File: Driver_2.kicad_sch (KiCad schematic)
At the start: 36 parts

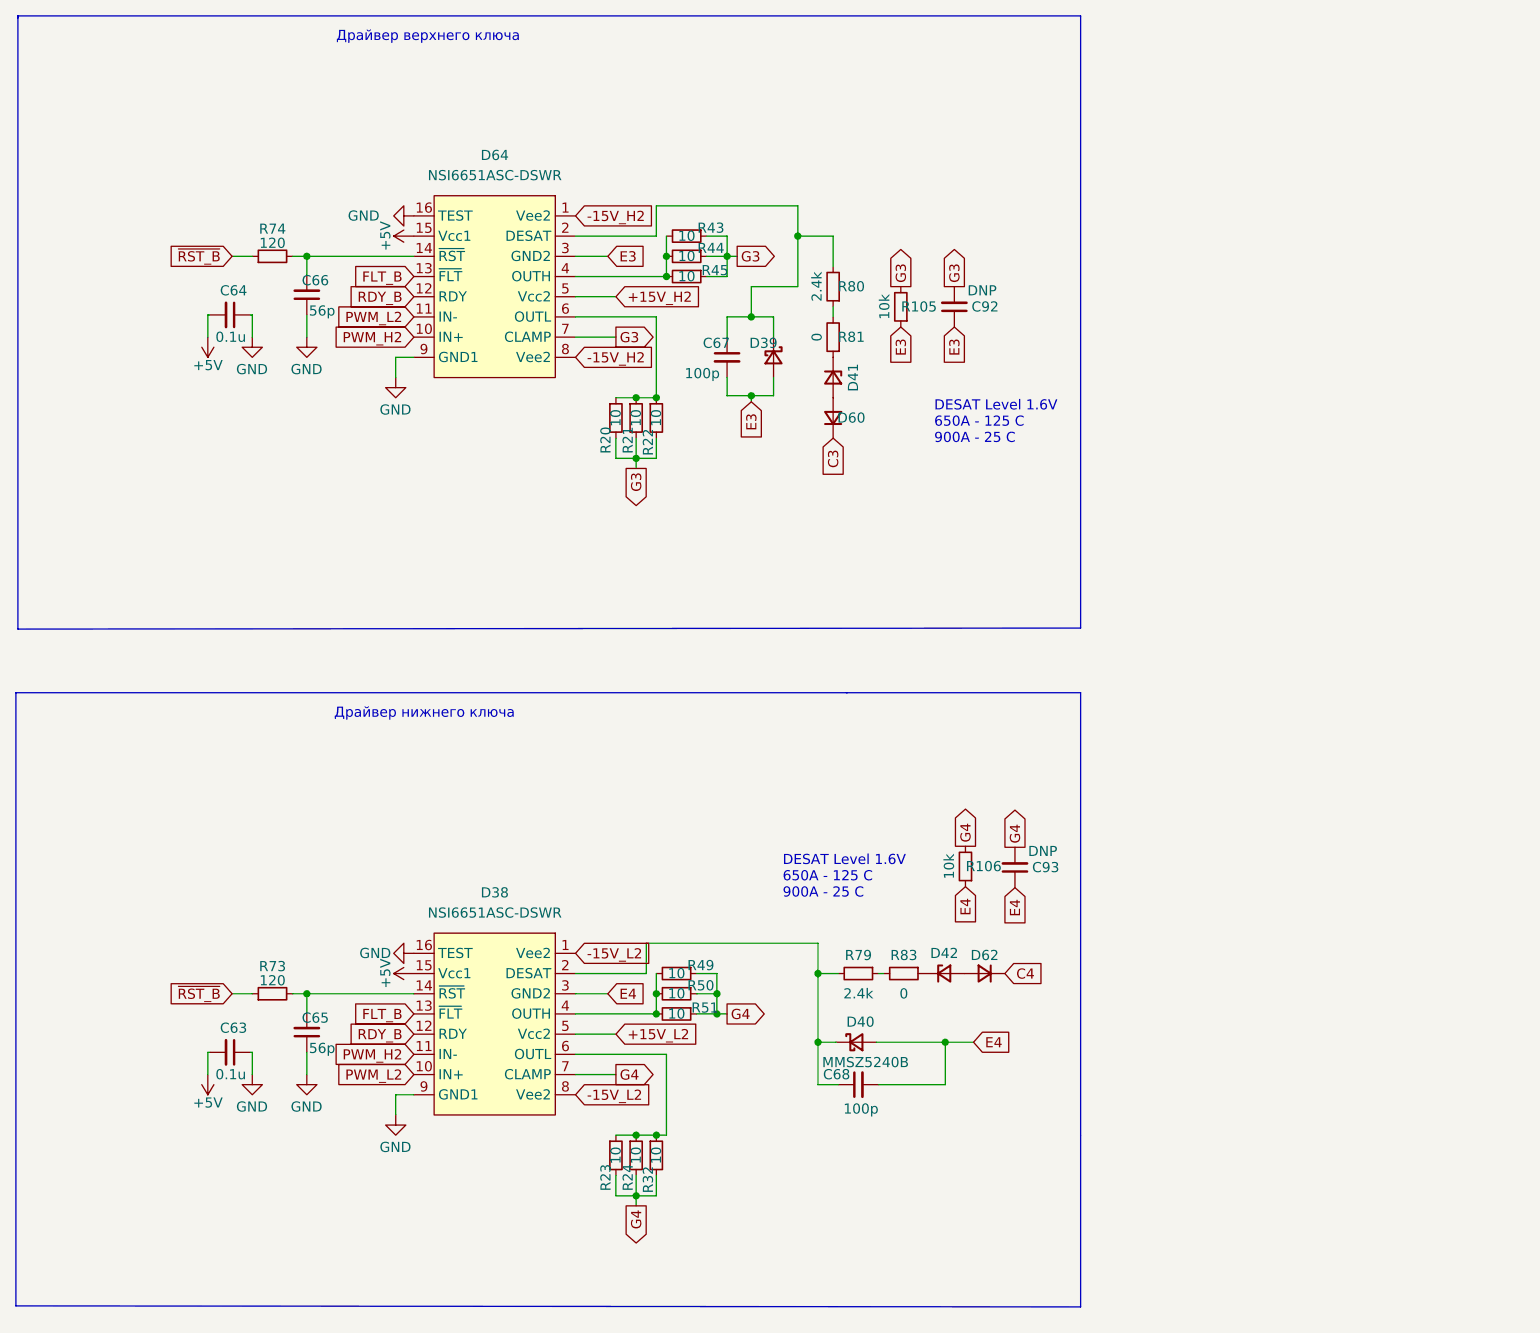
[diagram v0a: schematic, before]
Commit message: VER2.1: добавил СБ и 3D модели в доки
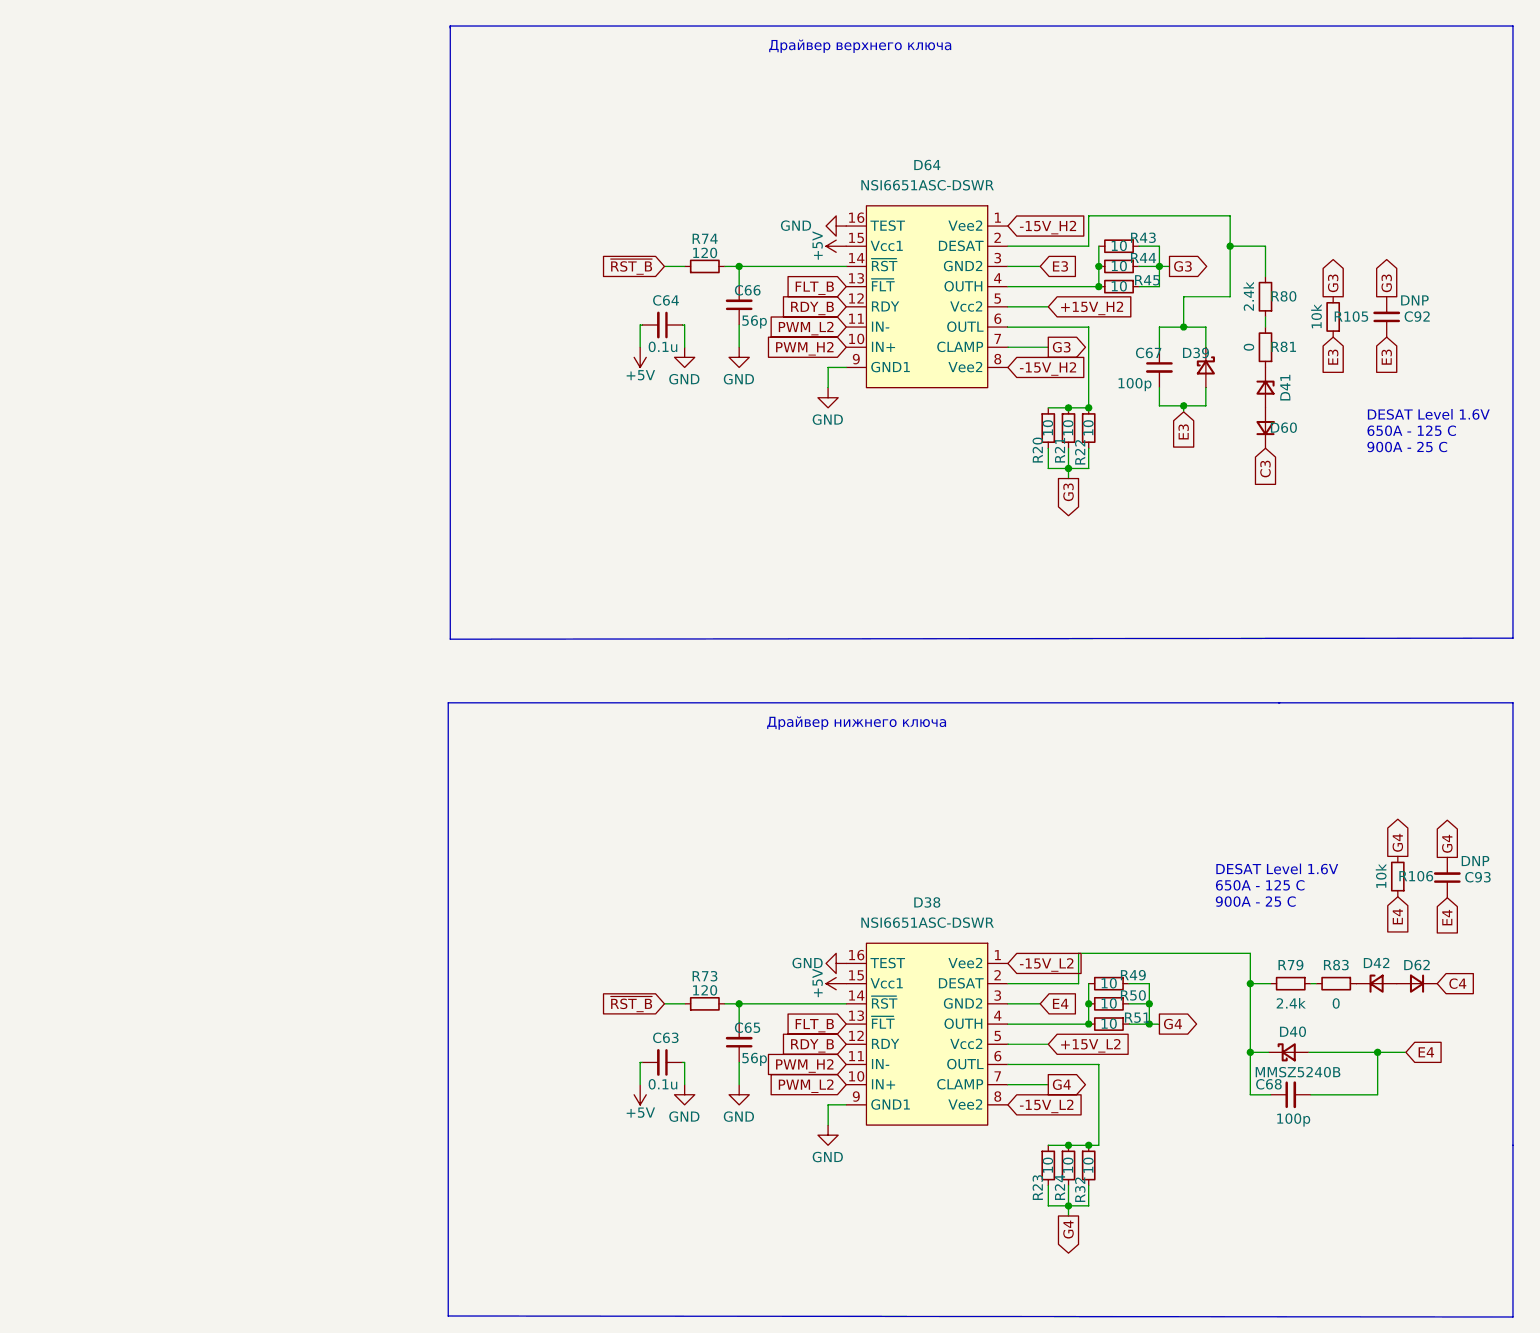
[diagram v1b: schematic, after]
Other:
- moved on the sheet: C63, C64, C65, C66, C67, C68, C92, C93, D38, D39, D40, D41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
